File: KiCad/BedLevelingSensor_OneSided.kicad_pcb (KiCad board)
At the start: 2 copper layers, 11.2 x 19.7 mm, 9 parts, among them J1 SOLENOID, J2 Sensor, J3 Input, U1 ATTINY15-1SC, U2 L9110

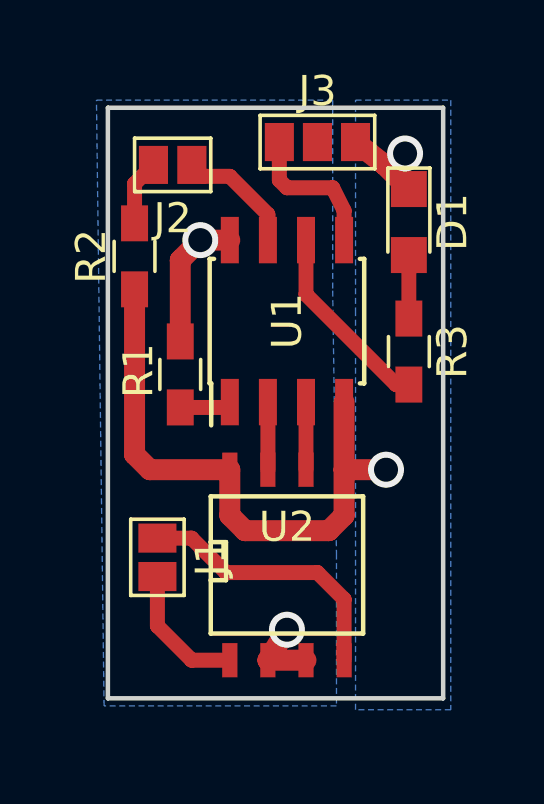
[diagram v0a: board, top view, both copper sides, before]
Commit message: Schematic/PCB adjust
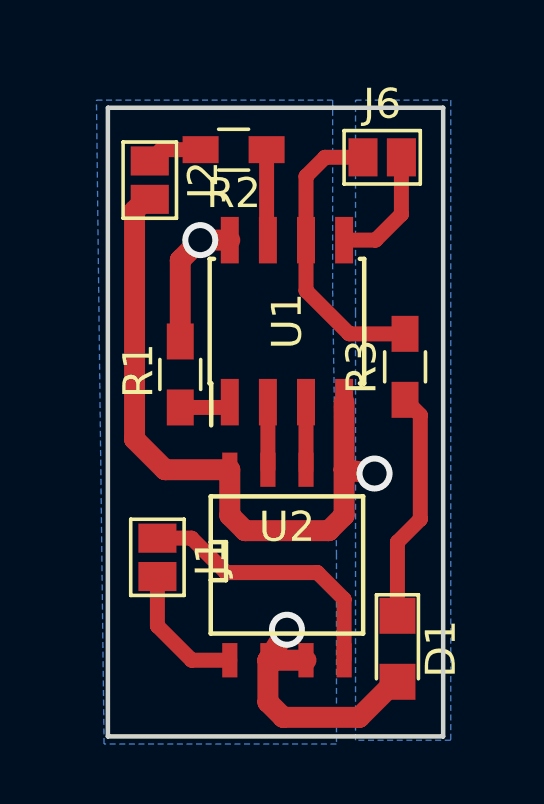
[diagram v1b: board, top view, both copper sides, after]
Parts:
- removed J3: Input, Connectors:GS3
- added J6: Inp_data, Connectors:GS2, F.Cu at (141.2, 107.8)
- R2: value 10K -> 1K
- moved D1 14.2 mm to (141.7, 124.2)
- moved R2 4.85 mm to (136.3, 107.6), turned to 180 degrees
- moved J2 0.92 mm to (133.5, 108.6), turned to 0 degrees
- moved R3 0.52 mm to (142.0, 114.8), turned to 90 degrees
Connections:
- net LED renamed MISO
- net Net-(R1-Pad2) renamed RST
- D1 pad 1: GND -> Net-(D1-Pad1)
- D1 pad 2: Net-(D1-Pad2) -> VCC
- J2 pad 2: Net-(J2-Pad2) -> GND
- R2 pad 1: GND -> SCK
- R2 pad 2: Net-(J2-Pad2) -> Net-(J2-Pad1)
- R3 pad 1: Net-(D1-Pad2) -> Net-(D1-Pad1)
- U1 pad 5: Net-(J3-Pad3) -> MOSI
- U1 pad 7: Net-(J2-Pad1) -> SCK
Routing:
- net Net-(D1-Pad1): track 0.00 -> 7.72 mm
- net VCC: track 7.46 -> 13.9 mm
- net Net-(J3-Pad3): track 4.99 -> 0.00 mm
- net MOSI: track 0.00 -> 4.17 mm
- net MISO: track 6.48 -> 9.87 mm
- net SCK: track 0.00 -> 3.03 mm
- net Net-(J2-Pad1): track 4.07 -> 1.85 mm
- net Net-(J2-Pad2): track 2.21 -> 0.00 mm
- net Net-(D1-Pad2): track 2.12 -> 0.00 mm
- net GND: track 23.0 -> 22.4 mm, vias 2 -> 1
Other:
- board size 11.2 x 19.7 mm -> 11.2 x 21 mm
